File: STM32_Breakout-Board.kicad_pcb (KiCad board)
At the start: 2 copper layers, 37 x 42 mm, 24 parts, among them U1 SPX3819M5-L-3-3, U2 STM32F042K6Tx, Y1 16MHz/10pF

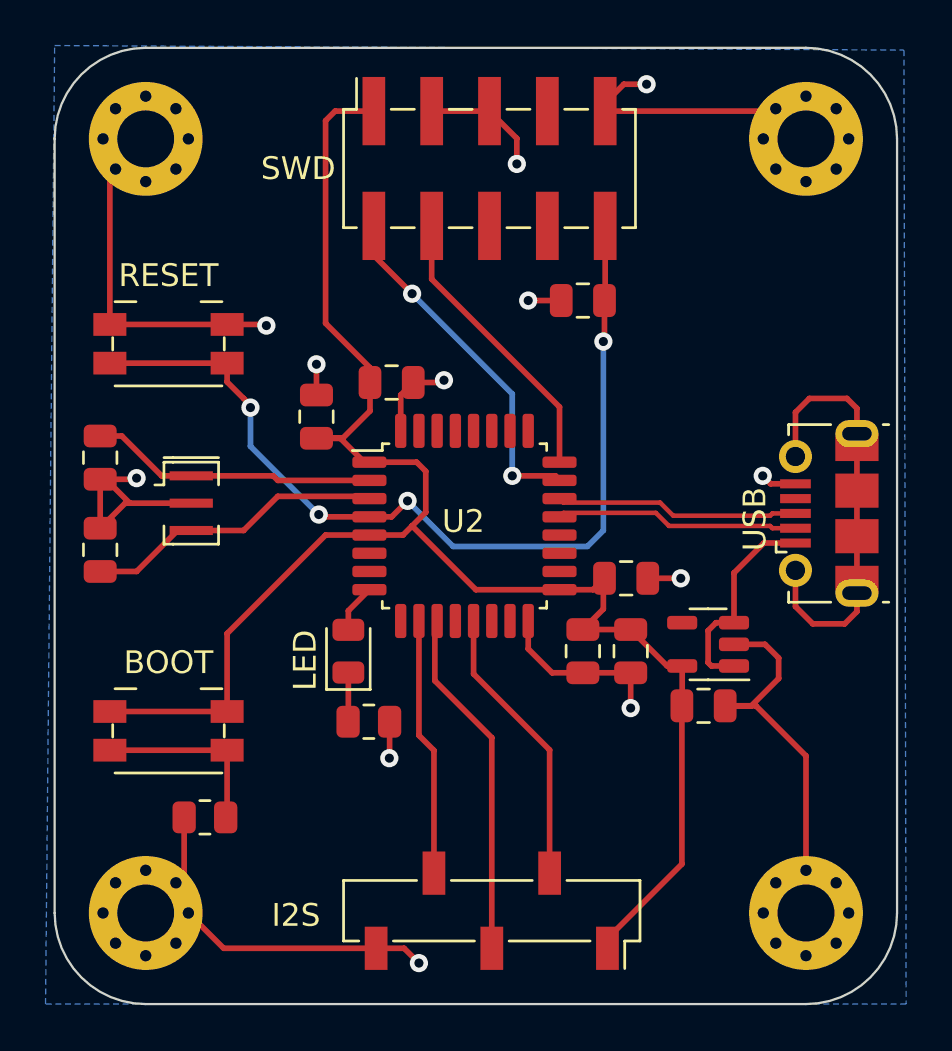
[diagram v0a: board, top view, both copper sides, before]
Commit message: Add files via upload
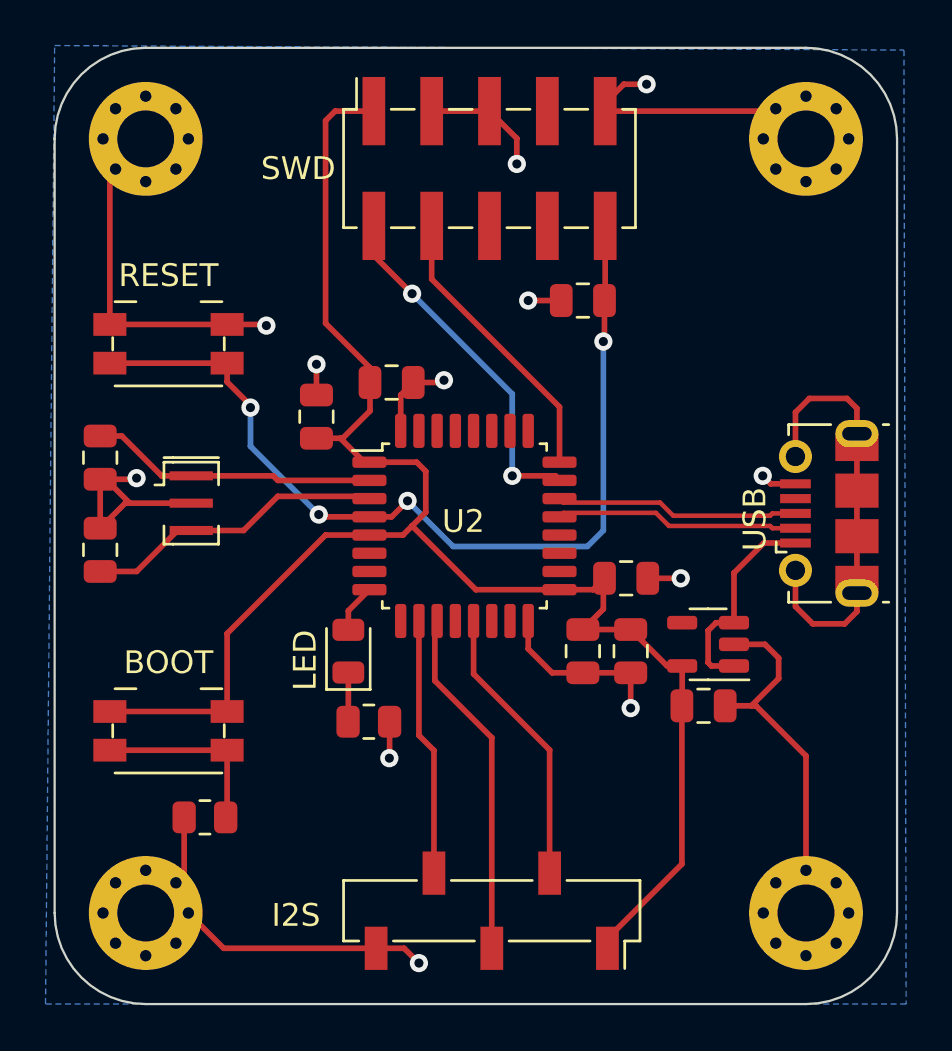
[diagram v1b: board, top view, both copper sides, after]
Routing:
- net GND: track 95.0 -> 93.6 mm
- net +3V3: track 76.7 -> 75.5 mm
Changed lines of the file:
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@@
   (segment (start 43.1 43.35) (end 43.1 44.65) (width 0.25) (layer "F.Cu") (net 1))
   (segment (start 26.575 49.15) (end 26.575 45.725) (width 0.25) (layer "F.Cu") (net 1))
-  (segment (start 31.55 37.15) (end 30.5 37.15) (width 0.25) (layer "F.Cu") (net 1))
   (segment (start 31.65 37.15) (end 32.85 35.95) (width 0.25) (layer "F.Cu") (net 1))
   (segment (start 32.85 34.05) (end 32.85 34.7) (width 0.25) (layer "F.Cu") (net 1))
@@
   (segment (start 33.02 22.78) (end 31.32 22.78) (width 0.25) (layer "F.Cu") (net 1))
   (segment (start 46.55 48.9) (end 46.55 55.85) (width 0.25) (layer "F.Cu") (net 1))
-  (segment (start 43.15 43.3) (end 43.1 43.35) (width 0.25) (layer "F.Cu") (net 1))
   (segment (start 43.28 59.12) (end 43.28 59.55) (width 0.25) (layer "F.Cu") (net 1))
   (segment (start 43.1 44.65) (end 42.2 45.55) (width 0.25) (layer "F.Cu") (net 1))
@@
   (segment (start 21.425 32.15) (end 21.425 25.575) (width 0.25) (layer "F.Cu") (net 2))
   (segment (start 21 41.1) (end 22.1 40) (width 0.25) (layer "F.Cu") (net 2))
-  (segment (start 49.6 48.9) (end 48.45 48.9) (width 0.25) (layer "F.Cu") (net 2))
   (segment (start 24.875 58) (end 26.425 59.55) (width 0.25) (layer "F.Cu") (net 2))
   (segment (start 26.575 32.15) (end 28.25 32.15) (width 0.25) (layer "F.Cu") (net 2))
@@
   (segment (start 24.6875 53.8) (end 24.6875 56.3125) (width 0.25) (layer "F.Cu") (net 2))
   (segment (start 44.3 49) (end 44.3 47.45) (width 0.25) (layer "F.Cu") (net 2))
-  (segment (start 21 38.95) (end 21.25 38.95) (width 0.25) (layer "F.Cu") (net 2))
   (segment (start 34.2 35.25) (end 34.75 34.7) (width 0.25) (layer "F.Cu") (net 2))
   (via (at 22.6 38.9) (size 0.8) (drill 0.4) (layers "F.Cu" "B.Cu") (net 2))
@@
   (segment (start 22.6 43) (end 24.4 41.2) (width 0.25) (layer "F.Cu") (net 4))
   (segment (start 43.15 31.1) (end 43.15 32.85) (width 0.25) (layer "F.Cu") (net 5))
-  (segment (start 27.3 35.4) (end 27.6 35.7) (width 0.25) (layer "F.Cu") (net 5))
+  (segment (start 26.575 34.675) (end 27.6 35.7) (width 0.25) (layer "F.Cu") (net 5))
   (segment (start 21.425 33.85) (end 26.575 33.85) (width 0.25) (layer "F.Cu") (net 5))
   (segment (start 32.825 40.6) (end 33.8 40.6) (width 0.25) (layer "F.Cu") (net 5))
@@
   (segment (start 27.6 35.7) (end 27.6 35.8) (width 0.25) (layer "F.Cu") (net 5))
   (segment (start 30.7 40.6) (end 30.6 40.5) (width 0.25) (layer "F.Cu") (net 5))
-  (segment (start 26.575 34.675) (end 27.3 35.4) (width 0.25) (layer "F.Cu") (net 5))
   (segment (start 43.15 32.85) (end 43.1 32.9) (width 0.25) (layer "F.Cu") (net 5))
   (segment (start 33.8 40.6) (end 34.5 39.9) (width 0.25) (layer "F.Cu") (net 5))
